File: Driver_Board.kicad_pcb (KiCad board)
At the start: 2 copper layers, 112.5 x 71.6 mm, 26 parts, among them J1 200, J2 100, J3 10, J4 Conn_01x04, J5 Conn_01x04, J6 Control

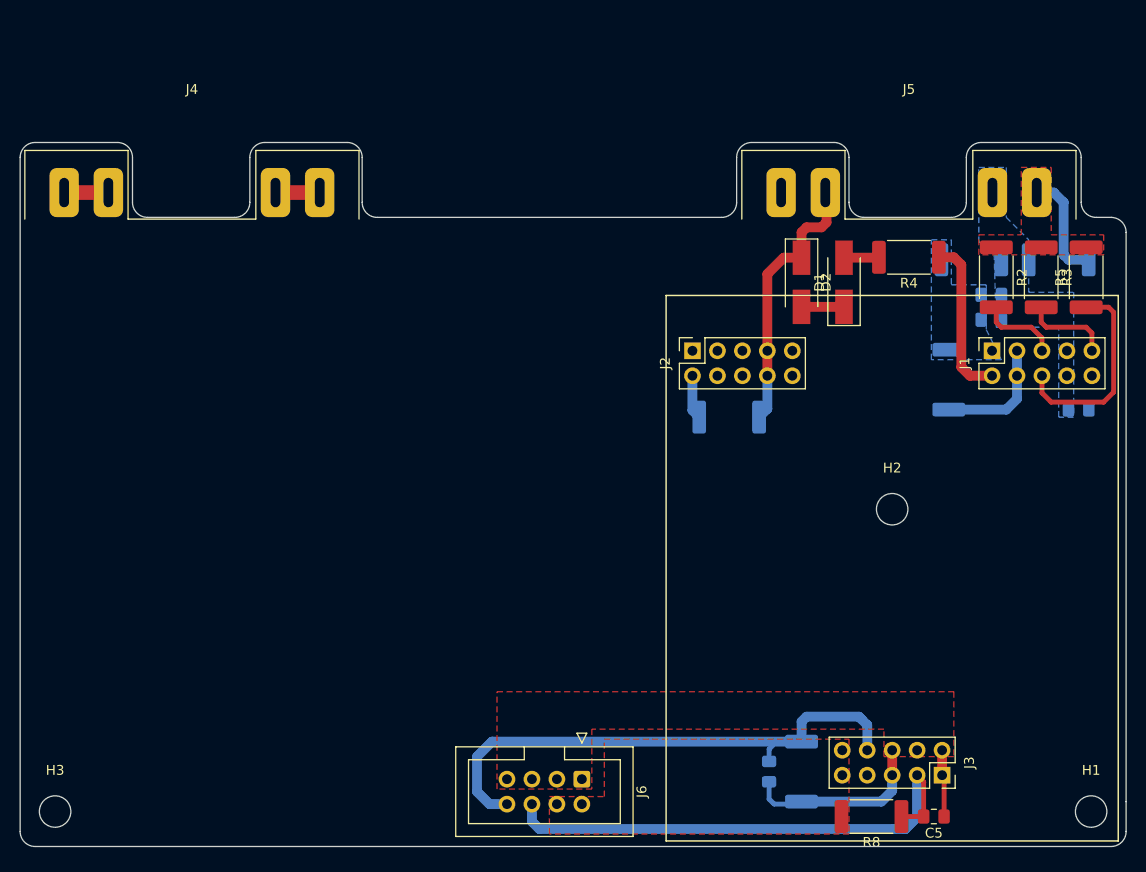
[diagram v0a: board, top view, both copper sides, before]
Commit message: Основа ADUM4135
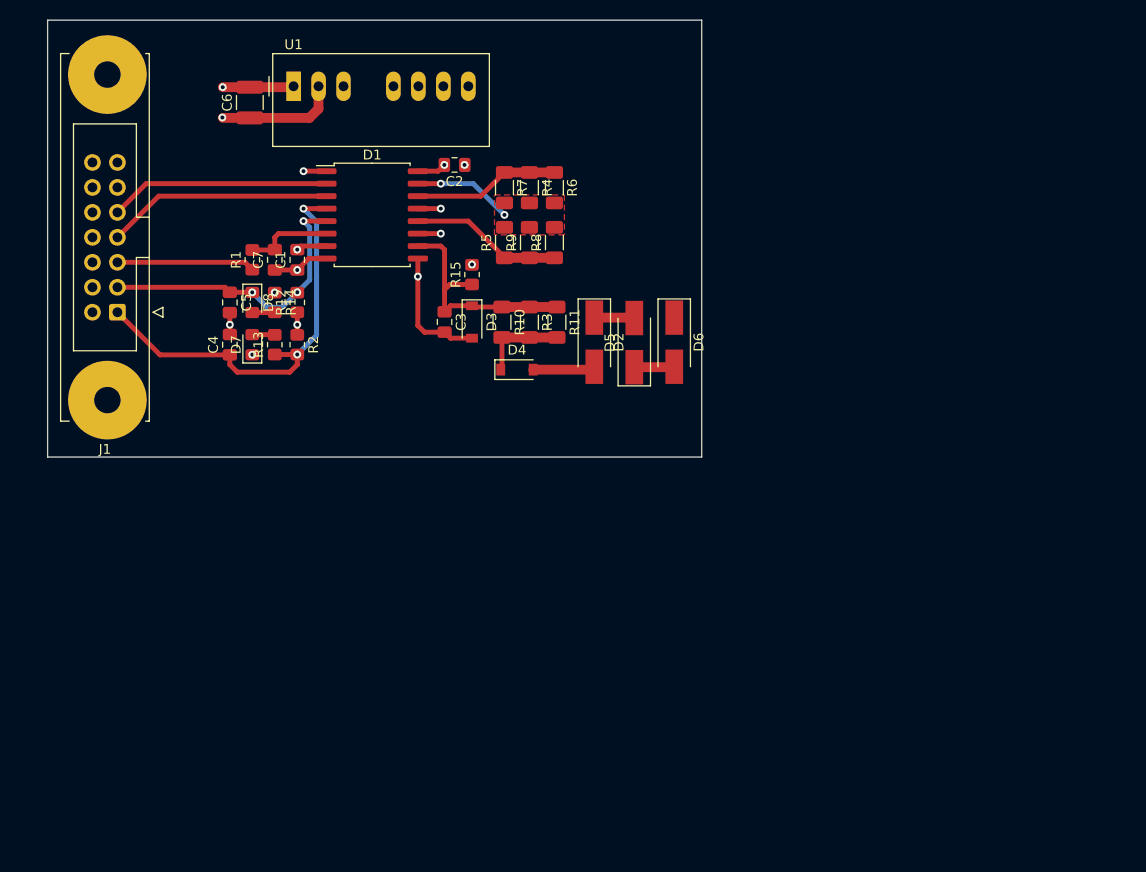
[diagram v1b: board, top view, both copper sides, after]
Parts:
- removed H1, H2, H3: MountingHole, MountingHole:MountingHole_3.2mm_M3
- removed J2: 100, Connector_PinSocket_2.54mm:PinSocket_2x05_P2.54mm_Vertical
- removed J3: 10, Connector_PinSocket_2.54mm:PinSocket_2x05_P2.54mm_Vertical
- removed J4, J5: Conn_01x04, IGBT_Modul:IGBT_Control
- removed J6: Control, Connector_IDC:IDC-Header_2x04_P2.54mm_Vertical
- added C6: 10u, Capacitor_SMD:C_1210_3225Metric_Pad1.33x2.70mm_HandSolder, F.Cu at (77.0, 62.7)
- added C7: 56p, Capacitor_SMD:C_0805_2012Metric_Pad1.18x1.45mm_HandSolder, F.Cu at (79.5, 78.7)
- added D3: BZT52C10-7-F, Diode_SMD:D_SOD-123, F.Cu at (99.6, 85.1)
- added D4: BZT52C10-7-F, Diode_SMD:D_SOD-123, F.Cu at (104.1, 89.9)
- added D5: MURS360T3G, Diode_SMD:D_SMA_Handsoldering, F.Cu at (116.1, 87.2)
- added D6: MURS360T3G, Diode_SMD:D_SMA_Handsoldering, F.Cu at (120.1, 87.1)
- added D7: LED_Small, LED_SMD:LED_0805_2012Metric_Pad1.15x1.40mm_HandSolder, F.Cu at (77.2, 87.4)
- added D8: LED_Small, LED_SMD:LED_0805_2012Metric_Pad1.15x1.40mm_HandSolder, F.Cu at (77.2, 83.1)
- added R12: 10k, Resistor_SMD:R_0805_2012Metric_Pad1.20x1.40mm_HandSolder, F.Cu at (81.8, 83.1)
- added R13: 380, Resistor_SMD:R_0805_2012Metric_Pad1.20x1.40mm_HandSolder, F.Cu at (79.5, 87.4)
- added R14: 500, Resistor_SMD:R_0805_2012Metric_Pad1.20x1.40mm_HandSolder, F.Cu at (79.5, 83.1)
- added R15: 2.2k, Resistor_SMD:R_0805_2012Metric_Pad1.20x1.40mm_HandSolder, F.Cu at (99.6, 80.2)
- added R9: 3.9, Resistor_SMD:R_1206_3216Metric_Pad1.30x1.75mm_HandSolder, F.Cu at (105.4, 77.0)
- added U1: TEC2-1213WI, Converter_DCDC:Converter_DCDC_TRACO_TMR-xxxx_THT, F.Cu at (81.4, 61.1)
- C1, C2: value C_Small -> 0.1u; moved to F.Cu
- C3: value CCFG -> 220p; moved to F.Cu
- C4: value 1n -> 0.1u; moved to F.Cu
- C5: value 100n -> 0.1u
- D1: value D_Small -> ADUM4135; footprint Diode_SMD:D_SMA_Handsoldering -> Package_SO:SOIC-16W_7.5x10.3mm_P1.27mm
- D2: value D_Small -> MURS360T3G
- J1: value 200 -> Conn_02x07_Odd_Even; footprint Connector_PinSocket_2.54mm:PinSocket_2x05_P2.54mm_Vertical -> Connector_IDC:IDC-Header_2x07-1MP_P2.54mm_Latch_Vertical
- R1: value 30.1k -> 120; footprint Resistor_SMD:R_2512_6332Metric_Pad1.40x3.35mm_HandSolder -> Resistor_SMD:R_0805_2012Metric_Pad1.20x1.40mm_HandSolder; moved to F.Cu
- R10: value 10k -> 12k; footprint Resistor_SMD:R_2512_6332Metric_Pad1.40x3.35mm_HandSolder -> Resistor_SMD:R_1206_3216Metric_Pad1.30x1.75mm_HandSolder; moved to F.Cu
- R11: value 0 -> 12k; footprint Resistor_SMD:R_2512_6332Metric_Pad1.40x3.35mm_HandSolder -> Resistor_SMD:R_1206_3216Metric_Pad1.30x1.75mm_HandSolder; moved to F.Cu
- R2: value RON -> 120; footprint Resistor_SMD:R_2512_6332Metric_Pad1.40x3.35mm_HandSolder -> Resistor_SMD:R_0805_2012Metric_Pad1.20x1.40mm_HandSolder
- R3: value 50 -> 12k; footprint Resistor_SMD:R_2512_6332Metric_Pad1.40x3.35mm_HandSolder -> Resistor_SMD:R_1206_3216Metric_Pad1.30x1.75mm_HandSolder
- R4: value 511 -> 3.9; footprint Resistor_SMD:R_2512_6332Metric_Pad1.40x3.35mm_HandSolder -> Resistor_SMD:R_1206_3216Metric_Pad1.30x1.75mm_HandSolder
- R5: value ROFF -> 3.9; footprint Resistor_SMD:R_2512_6332Metric_Pad1.40x3.35mm_HandSolder -> Resistor_SMD:R_1206_3216Metric_Pad1.30x1.75mm_HandSolder
- R6: value R1 -> 3.9; footprint Resistor_SMD:R_2512_6332Metric_Pad1.40x3.35mm_HandSolder -> Resistor_SMD:R_1206_3216Metric_Pad1.30x1.75mm_HandSolder; moved to F.Cu
- R7: value 10k -> 3.9; footprint Resistor_SMD:R_2512_6332Metric_Pad1.40x3.35mm_HandSolder -> Resistor_SMD:R_1206_3216Metric_Pad1.30x1.75mm_HandSolder; moved to F.Cu
- R8: value 30.1k -> 3.9; footprint Resistor_SMD:R_2512_6332Metric_Pad1.40x3.35mm_HandSolder -> Resistor_SMD:R_1206_3216Metric_Pad1.30x1.75mm_HandSolder
- moved J1 89.1 mm to (63.5, 84.1), turned to 180 degrees
- moved C5 88.7 mm to (74.9, 83.1), turned to -90 degrees
- moved R1 71.9 mm to (77.2, 78.7), turned to 90 degrees
- moved R2 71.4 mm to (81.8, 87.4)
- moved C1 70.9 mm to (81.8, 78.7), turned to 90 degrees
- moved C4 70.0 mm to (74.9, 87.4)
- moved C2 68.2 mm to (97.8, 69.1), turned to 180 degrees
- moved R8 66.7 mm to (108.0, 77.0), turned to 90 degrees
- moved R7 66.7 mm to (102.9, 71.4), turned to -90 degrees
- moved R5 59.3 mm to (102.9, 77.0)
- moved R10 57.0 mm to (102.6, 85.1), turned to -90 degrees
- moved C3 55.7 mm to (96.8, 85.1), turned to -90 degrees
- moved R3 52.3 mm to (105.4, 85.1)
- moved D1 48.5 mm to (89.4, 74.2), turned to 0 degrees
- moved R6 43.0 mm to (108.0, 71.4), turned to -90 degrees
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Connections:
- C1 pad 1: GNDPWR -> GNDA
- C1 pad 2: /CFG -> +5VD
- C2 pad 1: GNDPWR -> +15V
- C2 pad 2: Net-(C2-Pad2) -> E_IGBT
- C3 pad 1: /CFG -> Desat
- C3 pad 2: GNDPWR -> E_IGBT
- C4 pad 1: GND -> RDY
- C4 pad 2: /BOT_IN -> GNDA
- C5 pad 1: GND -> FLT
- C5 pad 2: /ERR_OUT -> GNDA
- D1 pad 1: Net-(D1-Pad1) -> GNDA
- D1 pad 2: Net-(D1-Pad2) -> IN+
- D2 pad 1: /E1 -> Net-(D2-Pad1)
- D2 pad 2: Net-(D1-Pad1) -> Net-(D2-Pad2)
- J1 pad 1: /CFG -> RDY
- J1 pad 10: Net-(C2-Pad2) -> GNDA
- J1 pad 2: Net-(J1-Pad2) -> GNDA
- J1 pad 3: /SEC_BOT -> FLT
- J1 pad 4: /SEC_BOT -> GNDA
- J1 pad 5: Net-(J1-Pad5) -> RST
- J1 pad 6: Net-(R5-Pad1) -> GNDA
- J1 pad 7: GNDPWR -> IN-
- J1 pad 8: GNDPWR -> GNDA
- J1 pad 9: Net-(J1-Pad9) -> IN+
- R1 pad 1: /CFG -> RST
- R1 pad 2: /SEC_BOT -> Net-(C7-Pad2)
- R10 pad 1: GNDPWR -> Desat
- R10 pad 2: /GATE -> Net-(D4-Pad1)
- R11 pad 1: Net-(J2-Pad2) -> Desat
- R11 pad 2: /E1 -> Net-(D4-Pad1)
- R2 pad 1: /GATE -> +5VD
- R2 pad 2: Net-(J1-Pad5) -> RDY
- R3 pad 1: /GATE -> Desat
- R3 pad 2: Net-(J1-Pad9) -> Net-(D4-Pad1)
- R4 pad 1: Net-(J1-Pad2) -> Net-(D1-Pad14)
- R4 pad 2: Net-(D1-Pad2) -> G_IGBT
- R5 pad 1: Net-(R5-Pad1) -> Net-(D1-Pad12)
- R5 pad 2: /GATE -> G_IGBT
- R6 pad 1: GNDPWR -> Net-(D1-Pad14)
- R6 pad 2: /CFG -> G_IGBT
- R7 pad 1: GND -> Net-(D1-Pad14)
- R7 pad 2: /BOT_IN -> G_IGBT
- R8 pad 1: /ERR_OUT -> Net-(D1-Pad12)
- R8 pad 2: +15V -> G_IGBT
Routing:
- net /BOT_IN: track 57.5 -> 0.00 mm
- net /ERR_OUT: track 52.8 -> 0.00 mm
- net RDY: track 0.00 -> 43.8 mm, vias 0 -> 2
- net FLT: track 0.00 -> 30.2 mm, vias 0 -> 3
- net /E1: track 27.7 -> 0.00 mm
- net GND: track 26.0 -> 0.00 mm
- net Desat: track 0.00 -> 23.9 mm
- net IN-: track 0.00 -> 23.0 mm
- net IN+: track 0.00 -> 22.5 mm
- net Net-(R5-Pad1): track 21.0 -> 0.00 mm
- net E_IGBT: track 0.00 -> 18.2 mm, vias 0 -> 3
- net GNDA: track 0.00 -> 17.5 mm, vias 0 -> 5
- net Net-(J1-Pad2): track 16.5 -> 0.00 mm
- net Net-(D1-Pad12): track 0.00 -> 16.2 mm
- net Net-(D1-Pad14): track 0.00 -> 15.1 mm
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- added copper zone on In1.Cu, net +15V
- added copper zone on In1.Cu, net +5VD
- added copper zone on In2.Cu, net E_IGBT
- added copper zone on In2.Cu, net GNDA
- added copper zone on F.Cu, net G_IGBT
- added copper zone on In1.Cu, net VAA
- removed copper zone on F.Cu, net +15V
- removed copper zone on B.Cu, net /CFG
- removed copper zone on F.Cu, net /GATE
- removed copper zone on F.Cu, net GND
- removed copper zone on B.Cu, net GNDPWR
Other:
- board size 112.5 x 71.6 mm -> 66.5 x 44.4 mm
- copper layers 2 -> 4
